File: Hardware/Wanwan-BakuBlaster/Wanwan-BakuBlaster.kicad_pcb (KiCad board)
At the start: 2 copper layers, 96 x 60.5 mm, 70 parts, among them Q1 BSS138, U1 RP2040-Zero, U2 PT8211, U3 TLV2372

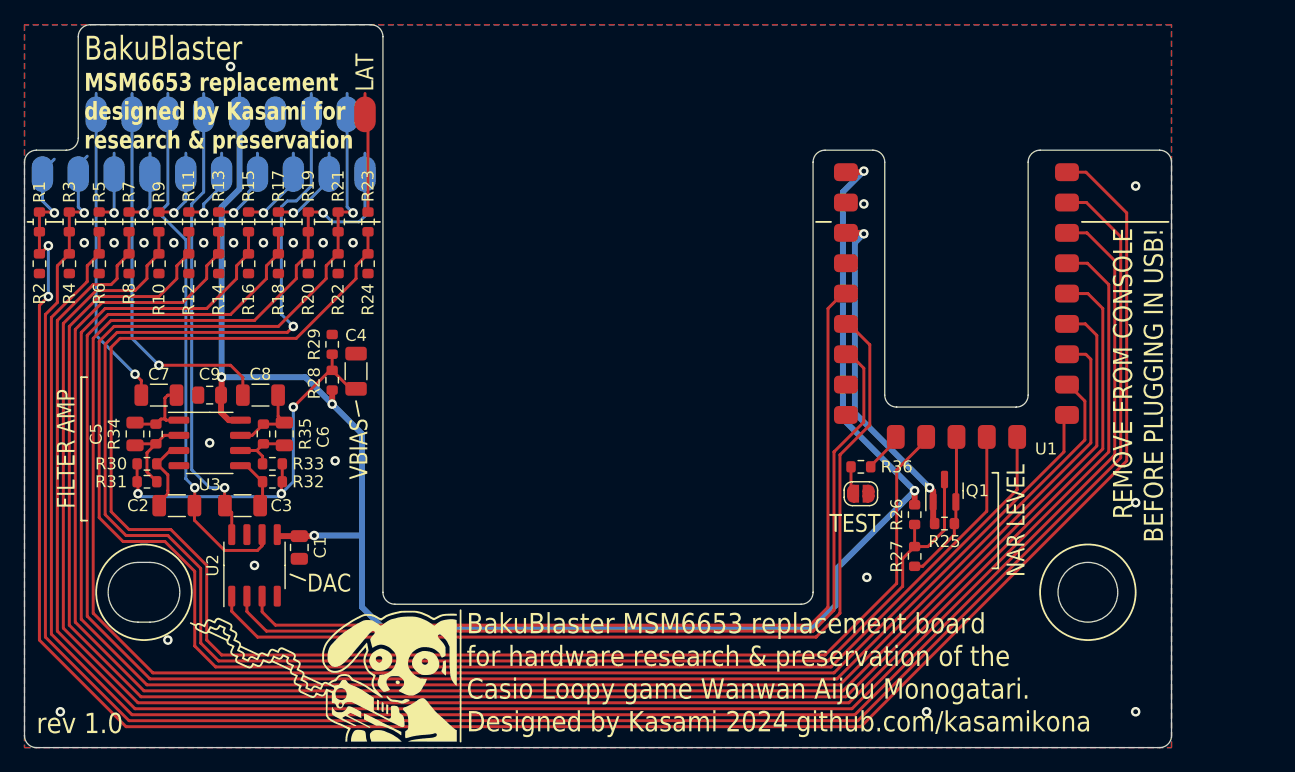
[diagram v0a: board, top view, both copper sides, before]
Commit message: Update hardware stuff
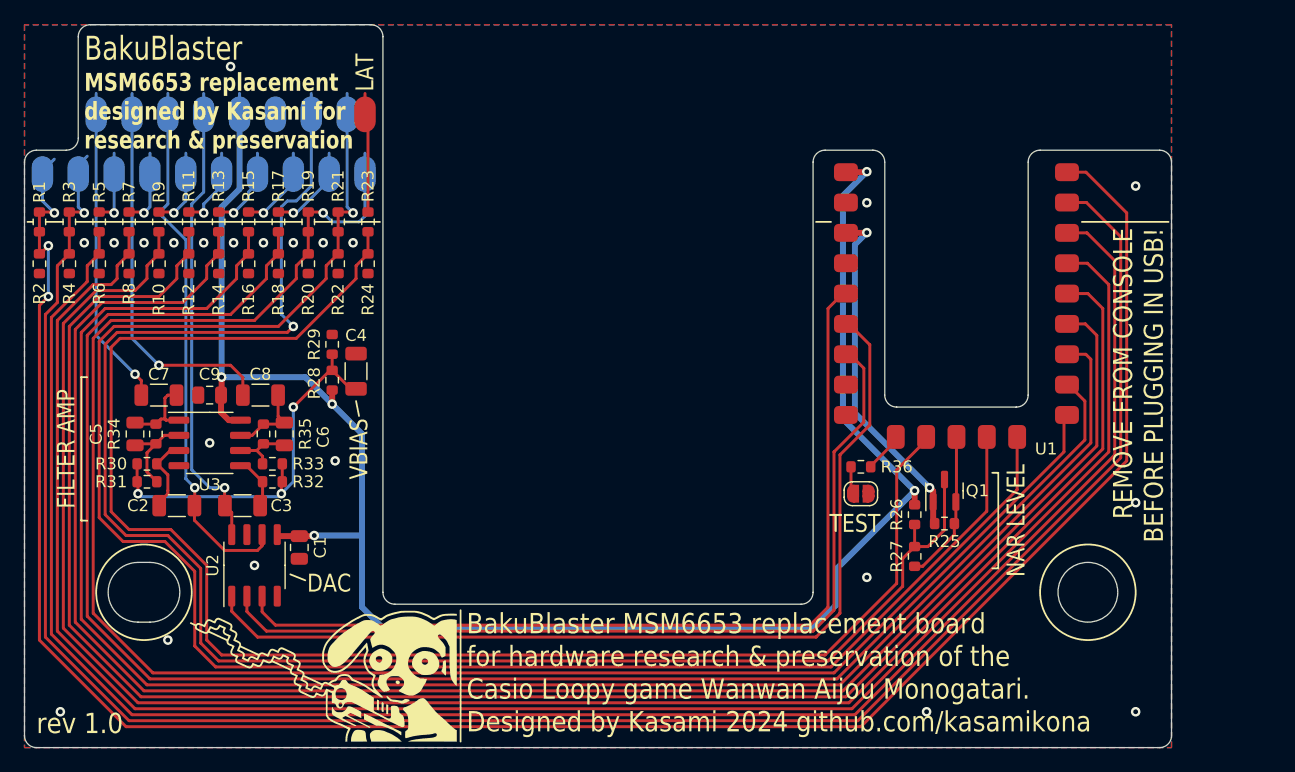
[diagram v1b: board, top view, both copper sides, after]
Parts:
- R1, R19, R21, R27, R3: value 1K -> DNP
- R25: value 2K2 -> DNP
